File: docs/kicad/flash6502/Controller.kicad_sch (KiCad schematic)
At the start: 8 parts

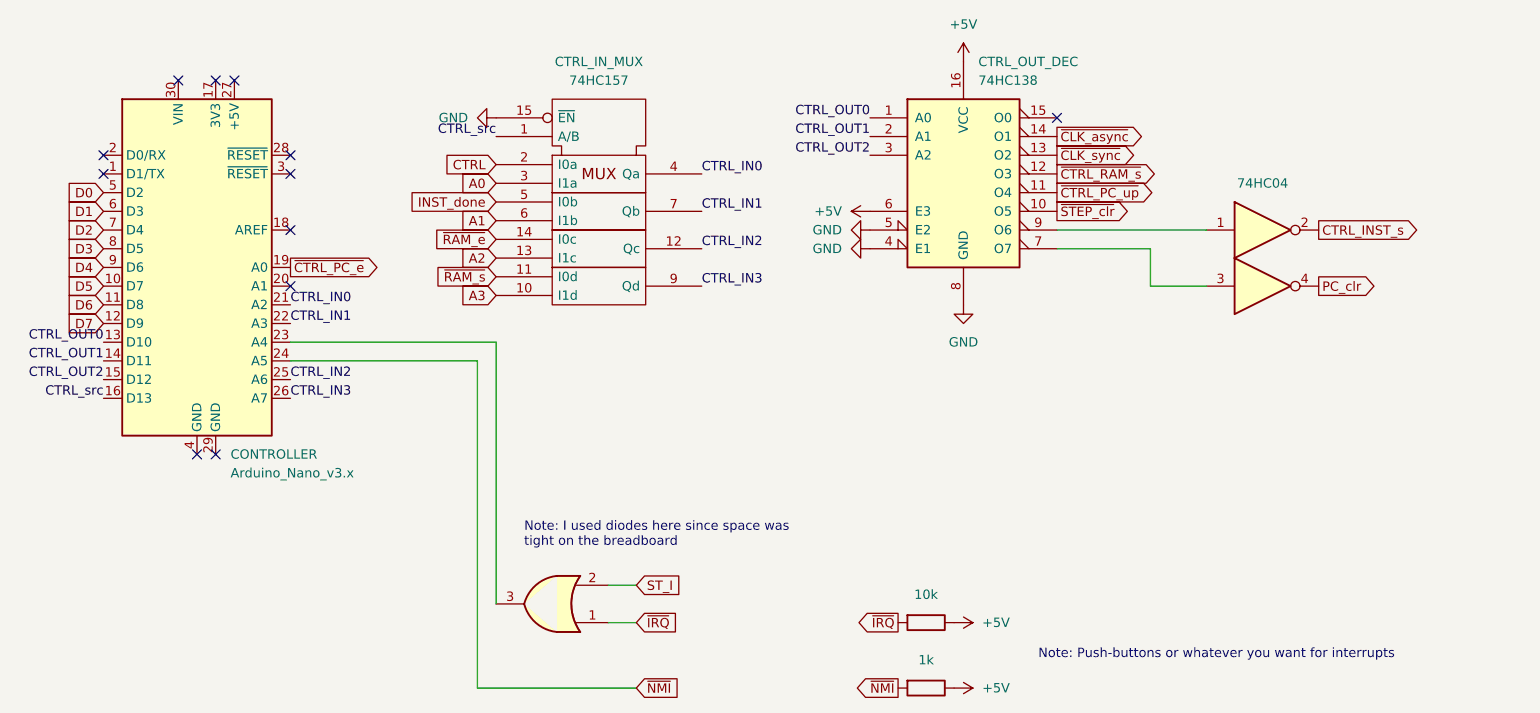
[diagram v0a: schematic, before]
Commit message: ok, docs
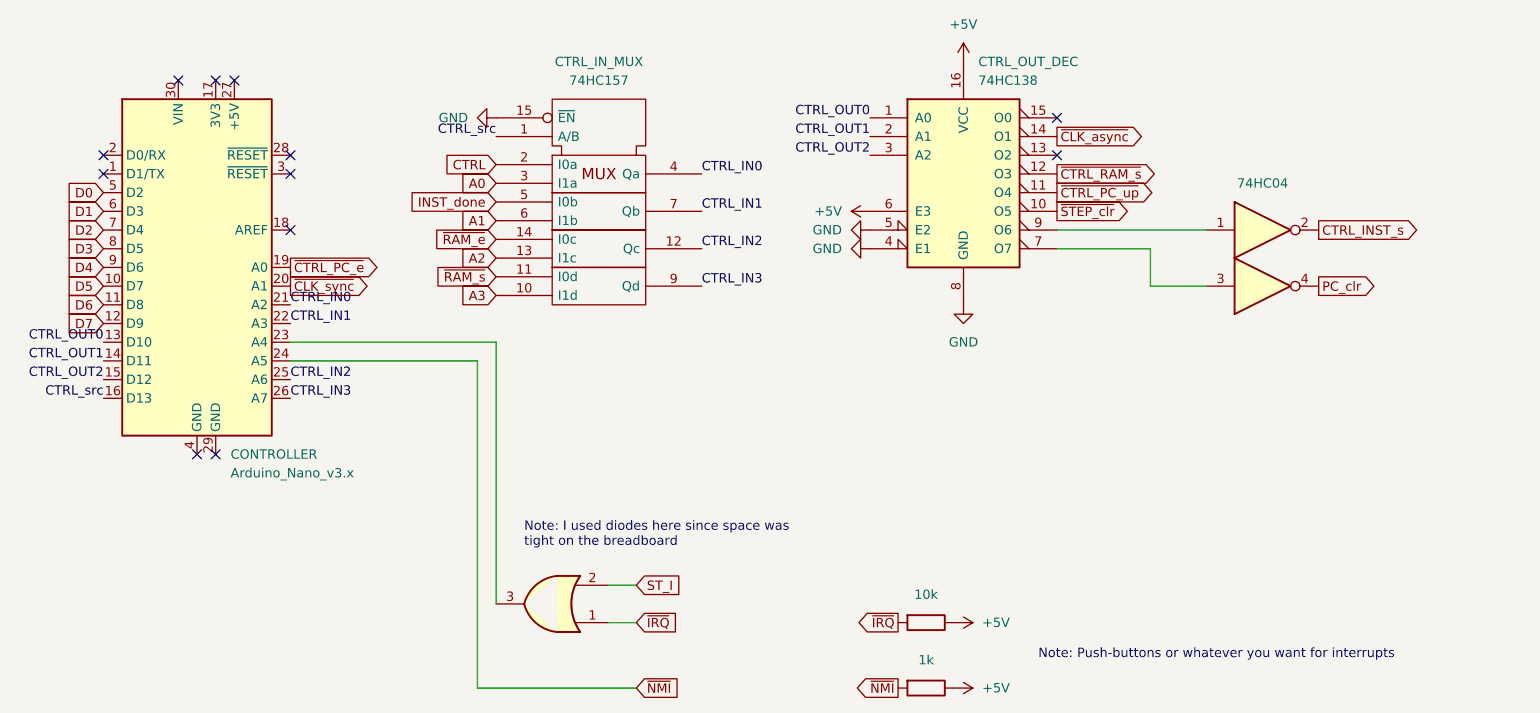
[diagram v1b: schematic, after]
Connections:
- net ~{CLK_sync}: now also CONTROLLER.20 (A1); no longer CTRL_OUT_DEC.13 (O2)
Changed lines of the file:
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@@
   (no_connect (at 35.56 44.45))
   (no_connect (at 60.96 52.07))
-  (no_connect (at 60.96 59.69))
+  (no_connect (at 165.1 41.91))
   (no_connect (at 165.1 36.83))
   (no_connect (at 50.8 31.75))
@@
     )
   )
+  (global_label "~{CLK_sync}" (shape output) (at 60.96 59.69 0) (fields_autoplaced)
+    (effects (font (size 1.27 1.27)) (justify left))
+    (property "Intersheet References" "${INTERSHEET_REFS}" (id 0) (at 72.1421 59.6106 0)
+      (effects (font (size 1.27 1.27)) (justify left) hide)
+    )
+  )
   (global_label "~{CTRL_PC_up}" (shape output) (at 165.1 46.99 0) (fields_autoplaced)
     (effects (font (size 1.27 1.27)) (justify left))
@@
     )
   )
-  (global_label "~{CLK_sync}" (shape output) (at 165.1 41.91 0) (fields_autoplaced)
-    (effects (font (size 1.27 1.27)) (justify left))
-    (property "Intersheet References" "${INTERSHEET_REFS}" (id 0) (at 176.2821 41.8306 0)
-      (effects (font (size 1.27 1.27)) (justify left) hide)
-    )
-  )

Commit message: ok
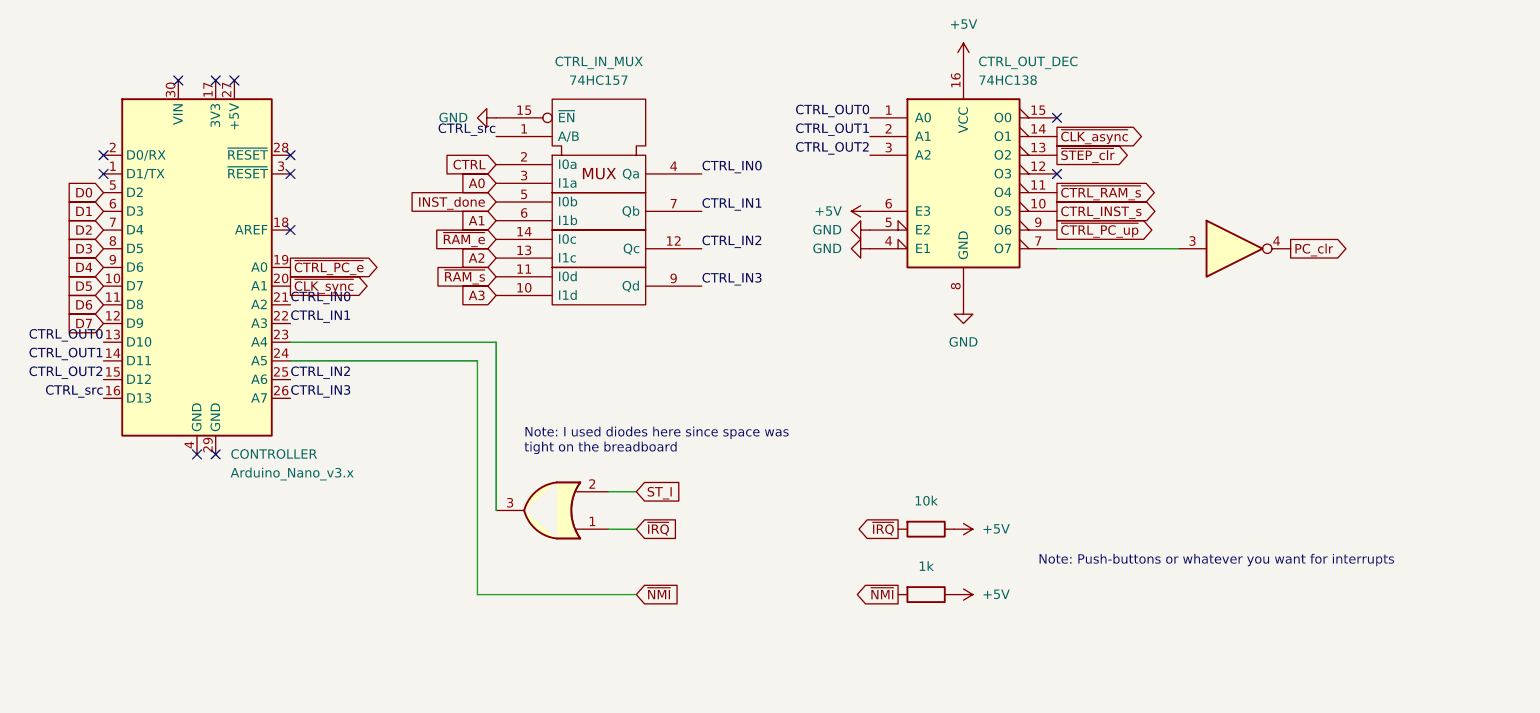
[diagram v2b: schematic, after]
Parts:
- removed CTRL_INST_s_NOT: 74HC04, symbol 74xx:74HC04
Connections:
- net CTRL_INST_s: now also CTRL_OUT_DEC.10 (O5)
- net ~{CTRL_PC_up}: now also CTRL_OUT_DEC.9 (O6); no longer CTRL_OUT_DEC.11 (O4)
- net ~{CTRL_RAM_s}: now also CTRL_OUT_DEC.11 (O4); no longer CTRL_OUT_DEC.12 (O3)
- net ~{STEP_clr}: now also CTRL_OUT_DEC.13 (O2); no longer CTRL_OUT_DEC.10 (O5)
